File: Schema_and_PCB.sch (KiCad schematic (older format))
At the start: 6 parts, among them SW1 PST-11A

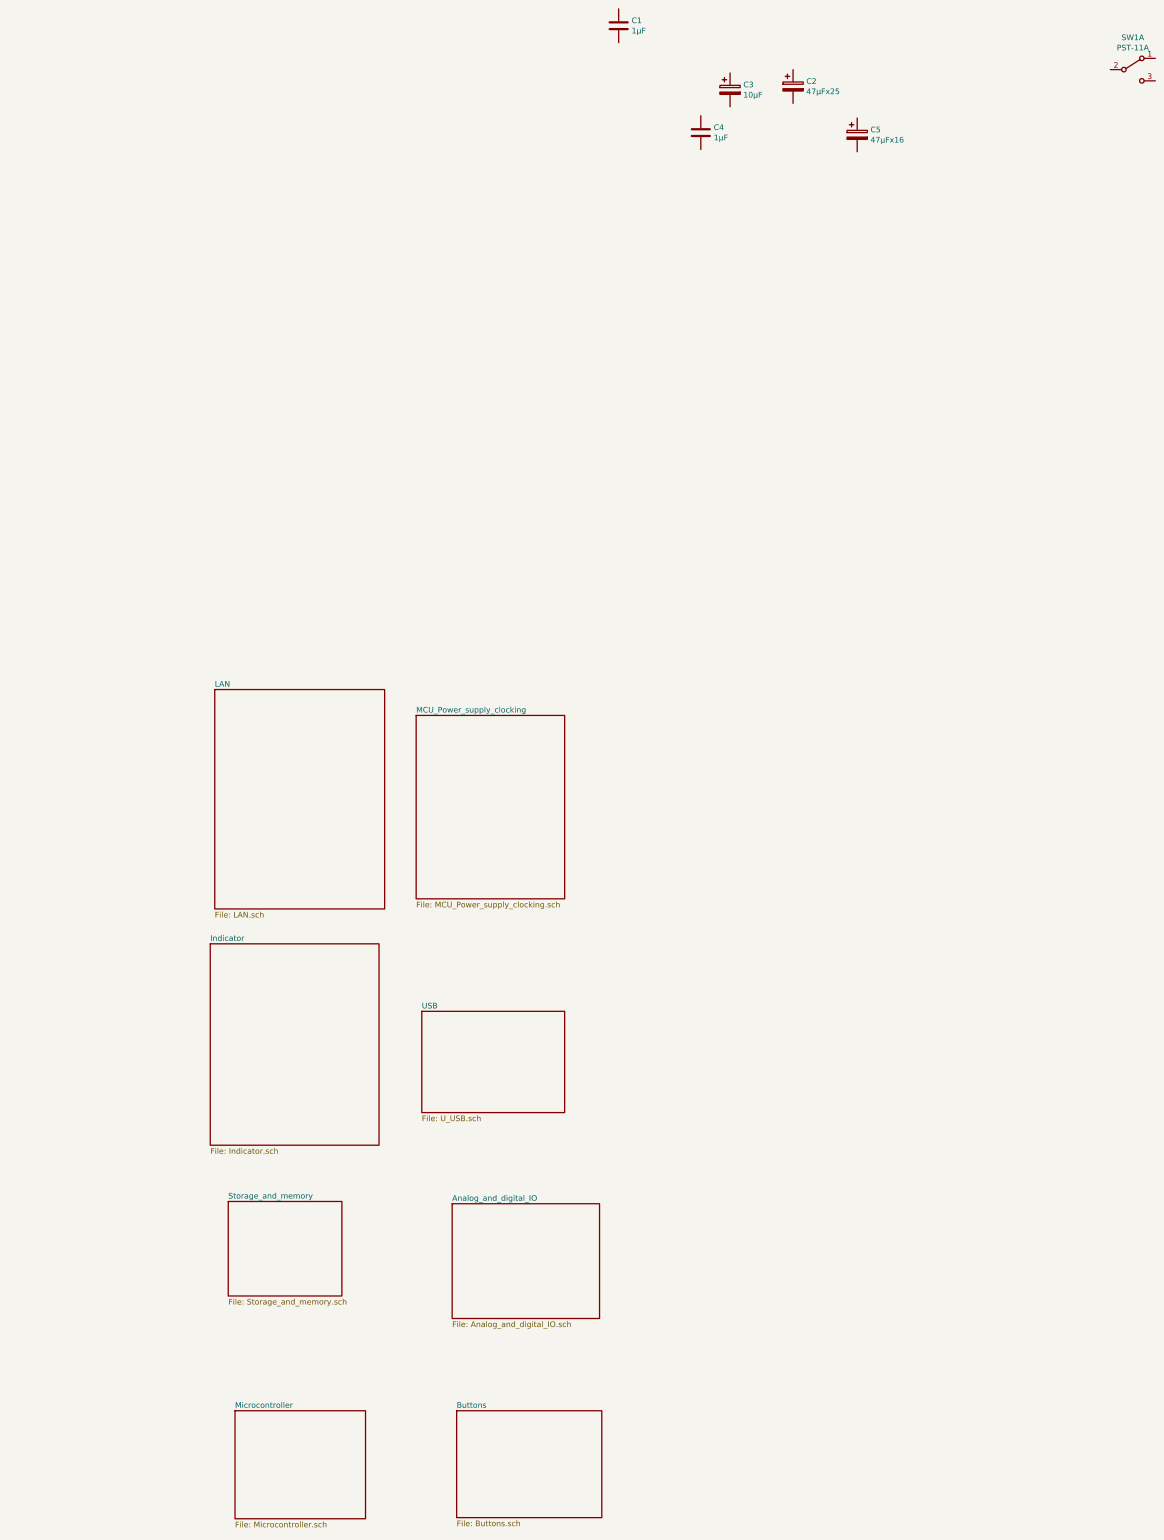
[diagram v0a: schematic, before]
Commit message: Probably pre-alpha version is done
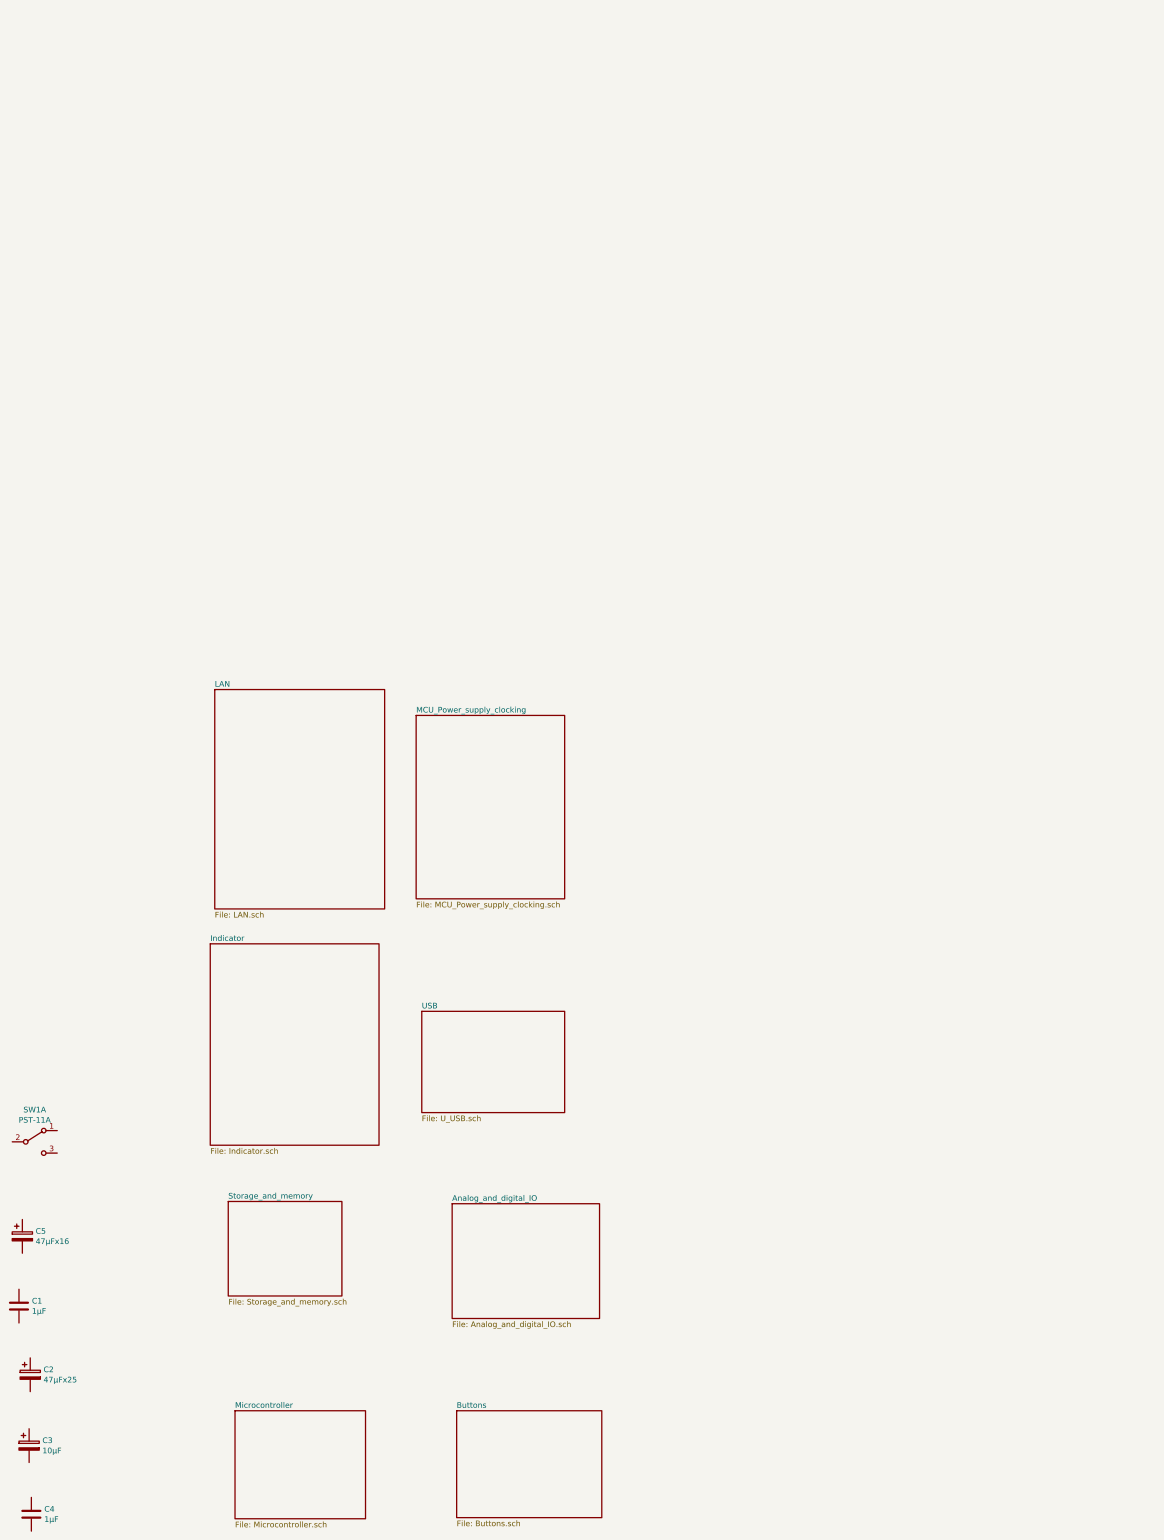
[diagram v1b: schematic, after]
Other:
- moved on the sheet: C1, C2, C3, C4, C5, SW1A
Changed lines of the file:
@@
 L Device:C C4
 U 1 1 606157F0
-P 5090 -1500
-F 0 "C4" H 5205 -1454 50  0000 L CNN
-F 1 "1µF" H 5205 -1545 50  0000 L CNN
-F 2 "Capacitor_SMD:C_0603_1608Metric_Pad1.08x0.95mm_HandSolder" H 5128 -1650 50  0001 C CNN
-F 3 "http://www.farnell.com/datasheets/2710676.pdf" H 5090 -1500 50  0001 C CNN
-F 4 "CL10B105KA8NNNC" H 5090 -1500 50  0001 C CNN "Type"
-	1    5090 -1500
+P -860 10780
+F 0 "C4" H -745 10826 50  0000 L CNN
+F 1 "1µF" H -745 10735 50  0000 L CNN
+F 2 "Capacitor_SMD:C_0603_1608Metric_Pad1.08x0.95mm_HandSolder" H -822 10630 50  0001 C CNN
+F 3 "http://www.farnell.com/datasheets/2710676.pdf" H -860 10780 50  0001 C CNN
+F 4 "CL10B105KA8NNNC" H -860 10780 50  0001 C CNN "Type"
+	1    -860 10780
 	1    0    0    -1
 $EndComp
@@
 L Device:CP C3
 U 1 1 6061539B
-P 5350 -1880
-F 0 "C3" H 5468 -1834 50  0000 L CNN
-F 1 "10µF" H 5468 -1925 50  0000 L CNN
-F 2 "Capacitor_Tantalum_SMD:CP_EIA-3216-10_Kemet-I" H 5388 -2030 50  0001 C CNN
-F 3 "http://www.mouser.com/ds/2/427/593d-239975.pdf" H 5350 -1880 50  0001 C CNN
-F 4 "593D106X9016A2TE3" H 5350 -1880 50  0001 C CNN "Type"
-	1    5350 -1880
+P -880 10170
+F 0 "C3" H -762 10216 50  0000 L CNN
+F 1 "10µF" H -762 10125 50  0000 L CNN
+F 2 "Capacitor_Tantalum_SMD:CP_EIA-3216-10_Kemet-I" H -842 10020 50  0001 C CNN
+F 3 "http://www.mouser.com/ds/2/427/593d-239975.pdf" H -880 10170 50  0001 C CNN
+F 4 "593D106X9016A2TE3" H -880 10170 50  0001 C CNN "Type"
+	1    -880 10170
 	1    0    0    -1
 $EndComp
@@
 L Device:CP C2
 U 1 1 6061A793
-P 5910 -1910
-F 0 "C2" H 6028 -1864 50  0000 L CNN
-F 1 "47µFx25" H 6028 -1955 50  0000 L CNN
-F 2 "Capacitor_Tantalum_SMD:CP_EIA-6032-28_Kemet-C_Pad2.25x2.35mm_HandSolder" H 5948 -2060 50  0001 C CNN
-F 3 "https://www.farnell.com/datasheets/1878216.pdf" H 5910 -1910 50  0001 C CNN
-F 4 "TR3D476K025C0150" H 5910 -1910 50  0001 C CNN "Type"
-	1    5910 -1910
+P -870 9540
+F 0 "C2" H -752 9586 50  0000 L CNN
+F 1 "47µFx25" H -752 9495 50  0000 L CNN
+F 2 "Capacitor_Tantalum_SMD:CP_EIA-6032-28_Kemet-C_Pad2.25x2.35mm_HandSolder" H -832 9390 50  0001 C CNN
+F 3 "https://www.farnell.com/datasheets/1878216.pdf" H -870 9540 50  0001 C CNN
+F 4 "TR3D476K025C0150" H -870 9540 50  0001 C CNN "Type"
+	1    -870 9540
 	1    0    0    -1
 $EndComp
@@
 L Device:C C1
 U 1 1 60633F0C
-P 4360 -2450
-F 0 "C1" H 4475 -2404 50  0000 L CNN
-F 1 "1µF" H 4475 -2495 50  0000 L CNN
-F 2 "Capacitor_SMD:C_0603_1608Metric_Pad1.08x0.95mm_HandSolder" H 4398 -2600 50  0001 C CNN
-F 3 "https://www.farnell.com/datasheets/2048520.pdf" H 4360 -2450 50  0001 C CNN
-F 4 "GRM188R7YA105KA12D" H 4360 -2450 50  0001 C CNN "Type"
-	1    4360 -2450
+P -970 8930
+F 0 "C1" H -855 8976 50  0000 L CNN
+F 1 "1µF" H -855 8885 50  0000 L CNN
+F 2 "Capacitor_SMD:C_0603_1608Metric_Pad1.08x0.95mm_HandSolder" H -932 8780 50  0001 C CNN
+F 3 "https://www.farnell.com/datasheets/2048520.pdf" H -970 8930 50  0001 C CNN
+F 4 "GRM188R7YA105KA12D" H -970 8930 50  0001 C CNN "Type"
+	1    -970 8930
 	1    0    0    -1
 $EndComp
@@
 L Device:CP C5
 U 1 1 60634752
-P 6480 -1480
-F 0 "C5" H 6598 -1434 50  0000 L CNN
-F 1 "47µFx16" H 6598 -1525 50  0000 L CNN
-F 2 "Capacitor_Tantalum_SMD:CP_EIA-7343-31_Kemet-D_Pad2.25x2.55mm_HandSolder" H 6518 -1630 50  0001 C CNN
-F 3 "https://www.farnell.com/datasheets/1995953.pdf" H 6480 -1480 50  0001 C CNN
-F 4 "593D476X9016D2TE3" H 6480 -1480 50  0001 C CNN "Type"
-	1    6480 -1480
+P -940 8310
+F 0 "C5" H -822 8356 50  0000 L CNN
+F 1 "47µFx16" H -822 8265 50  0000 L CNN
+F 2 "Capacitor_Tantalum_SMD:CP_EIA-7343-31_Kemet-D_Pad2.25x2.55mm_HandSolder" H -902 8160 50  0001 C CNN
+F 3 "https://www.farnell.com/datasheets/1995953.pdf" H -940 8310 50  0001 C CNN
+F 4 "593D476X9016D2TE3" H -940 8310 50  0001 C CNN "Type"
+	1    -940 8310
 	1    0    0    -1
 $EndComp
@@
 L Switch:SW_DPDT_x2 SW1
 U 1 1 6063E7A3
-P 8930 -2060
-F 0 "SW1" H 8930 -1775 50  0000 C CNN
-F 1 "PST-11A" H 8930 -1866 50  0000 C CNN
-F 2 "" H 8930 -2060 50  0001 C CNN
-F 3 "https://www.terraelectronica.ru/product/45953" H 8930 -2060 50  0001 C CNN
-	1    8930 -2060
+P -830 7470
+F 0 "SW1" H -830 7755 50  0000 C CNN
+F 1 "PST-11A" H -830 7664 50  0000 C CNN
+F 2 "" H -830 7470 50  0001 C CNN
+F 3 "https://www.terraelectronica.ru/product/45953" H -830 7470 50  0001 C CNN
+	1    -830 7470
 	1    0    0    -1
 $EndComp
